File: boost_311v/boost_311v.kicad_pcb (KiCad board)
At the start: 2 copper layers, 44 parts, among them Q1 BC556, Q2 PN2222A, Q3 PN2222A, U1 NE555, U2 4N25, U3 4N25, U4 TL081, U5 NE555

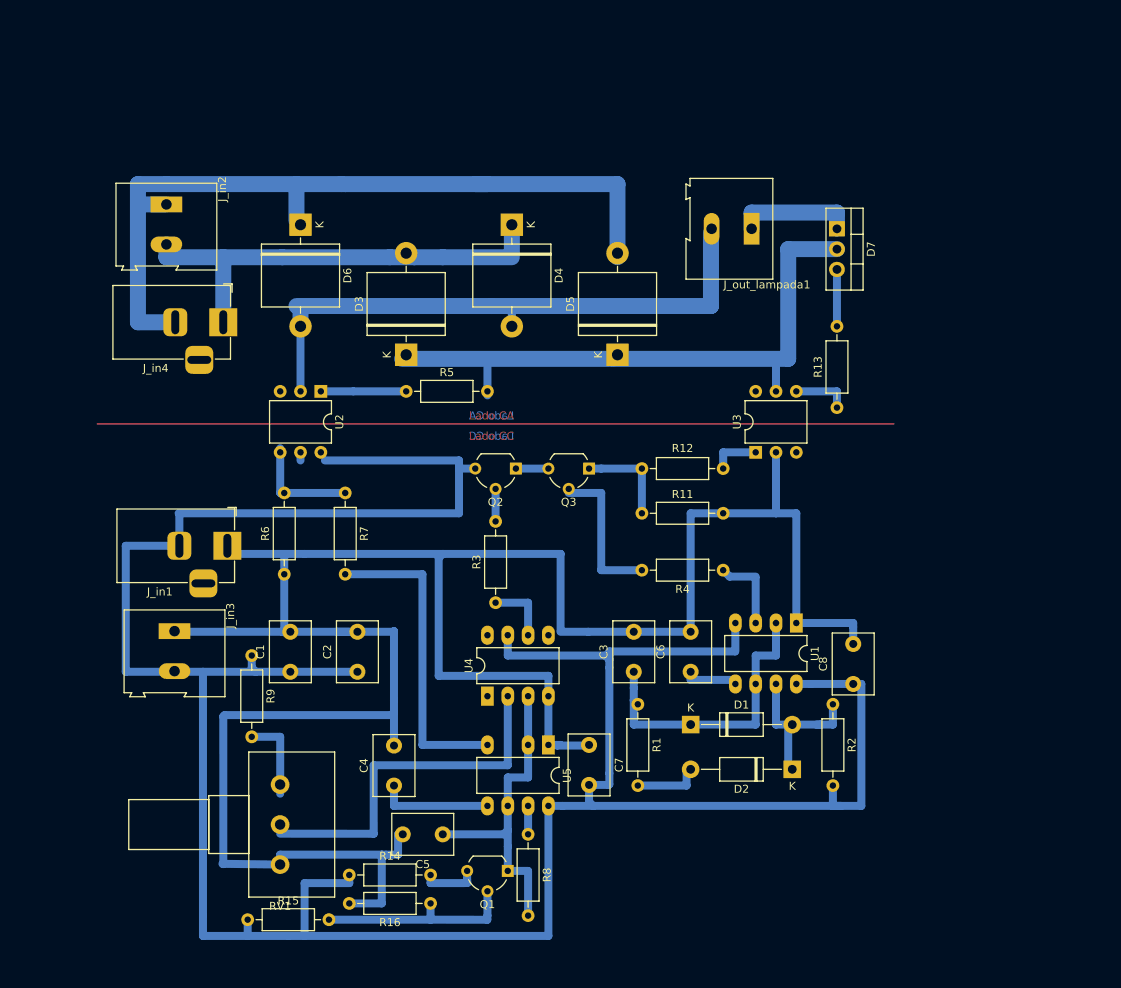
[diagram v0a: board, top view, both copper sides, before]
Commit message: Up pcb
Signed-off-by: fgl27 <fglfgl27@gmail.com>
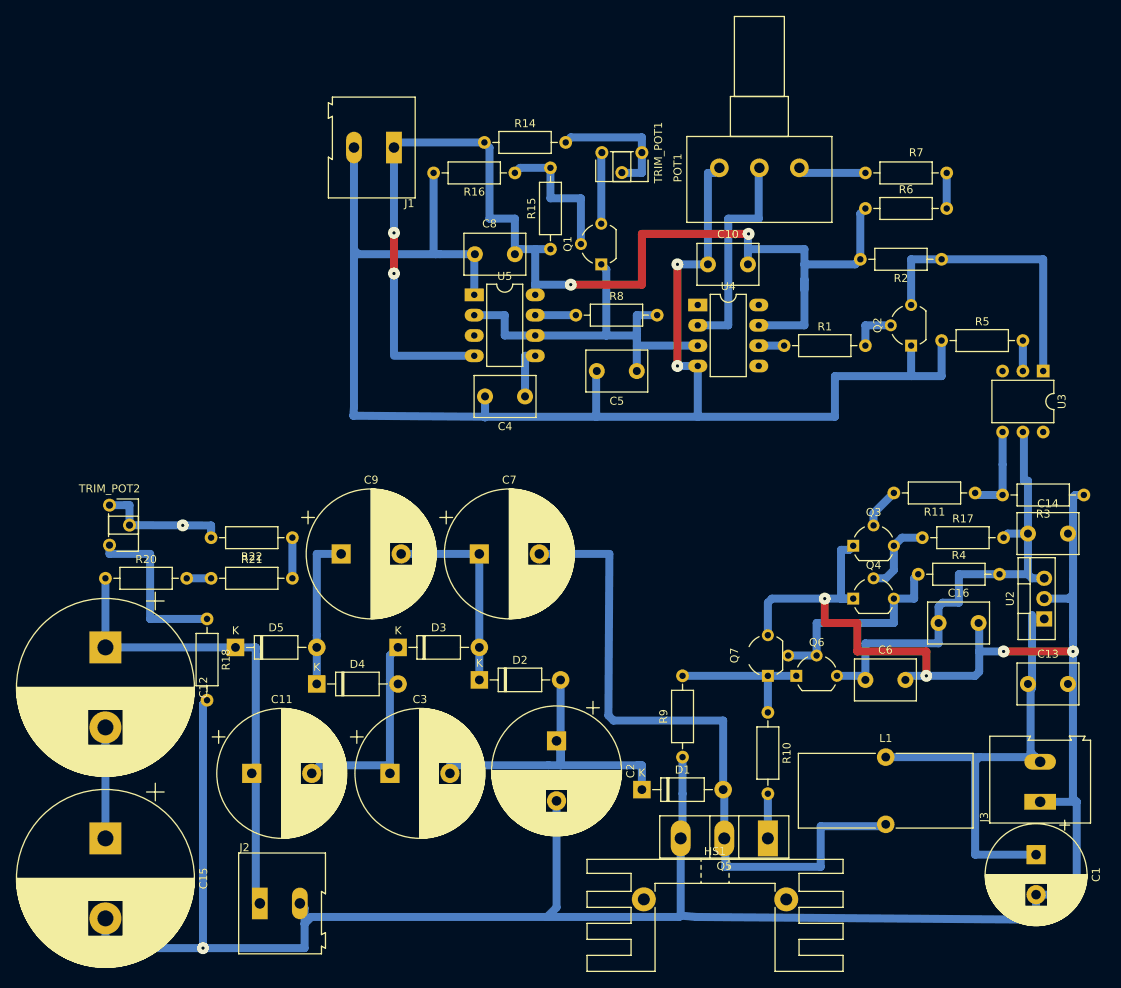
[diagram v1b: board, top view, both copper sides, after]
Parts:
- removed D6: DIODE, Diode_THT:D_5KP_P12.70mm_Horizontal
- removed D7: BT151, Package_TO_SOT_THT:TO-220-3_Vertical
- removed J_in1, J_in4: Screw_Terminal_01x02, Connector_BarrelJack:BarrelJack_Horizontal
- removed J_in2, J_in3, J_out_lampada1: Screw_Terminal_01x02, TerminalBlock:TerminalBlock_Altech_AK300-2_P5.00mm
- removed R12, R13: 1k, Resistor_THT:R_Axial_DIN0207_L6.3mm_D2.5mm_P10.16mm_Horizontal
- removed RV1: POT_10k, Potentiometer_THT:Potentiometer_Alps_RK163_Single_Horizontal
- removed U1: NE555, Package_DIP:DIP-8_W7.62mm_LongPads
- added C10: 100nF, Capacitor_THT:C_Disc_D7.5mm_W5.0mm_P5.00mm, F.Cu at (127.1, 98.4)
- added C11: 100µF_200V, Capacitor_THT:CP_Radial_D16.0mm_P7.50mm, F.Cu at (70.1, 162.1)
- added C12: 200µF_200V, Capacitor_THT:CP_Radial_D22.0mm_P10.00mm_SnapIn, F.Cu at (51.8, 146.3)
- added C13: 10µF, Capacitor_THT:C_Disc_D7.5mm_W5.0mm_P5.00mm, F.Cu at (167.1, 150.9)
- added C14: 100nF, Capacitor_THT:C_Disc_D7.5mm_W5.0mm_P5.00mm, F.Cu at (167.1, 132.1)
- added C15: 200µF_200V, Capacitor_THT:CP_Radial_D22.0mm_P10.00mm_SnapIn, F.Cu at (51.8, 170.2)
- added C16: 100nF, Capacitor_THT:C_Disc_D7.5mm_W5.0mm_P5.00mm, F.Cu at (156.0, 143.3)
- added C9: 100µF_200V, Capacitor_THT:CP_Radial_D16.0mm_P7.50mm, F.Cu at (81.3, 134.6)
- added HS1: Heatsink, Heatsink:Heatsink_Stonecold_HS-132_32x14mm_2xFixation1.5mm, F.Cu at (128.0, 177.8)
- added J1: Vin_cnt, TerminalBlock:TerminalBlock_Altech_AK300-2_P5.00mm, F.Cu at (87.9, 83.8)
- added J2: VO, TerminalBlock:TerminalBlock_Altech_AK300-2_P5.00mm, F.Cu at (71.1, 178.3)
- added J3: Vin_boost, TerminalBlock:TerminalBlock_Altech_AK300-2_P5.00mm, F.Cu at (168.7, 165.6)
- added L1: 20µH, Inductor_THT:L_Toroid_Vertical_L21.6mm_W9.1mm_P8.40mm_Bourns_5700, F.Cu at (149.4, 160.0)
- added POT1: 200kΩ, Potentiometer_THT:Potentiometer_Alps_RK163_Single_Horizontal, F.Cu at (138.6, 86.4)
- added Q4: PN2222A, Package_TO_SOT_THT:TO-92_Wide, F.Cu at (145.3, 140.2)
- added Q5: IRFP260, Package_TO_SOT_THT:TO-247-3_Vertical, F.Cu at (134.6, 170.2)
- added Q6: 2N3904, Package_TO_SOT_THT:TO-92_Wide, F.Cu at (138.2, 149.9)
- added Q7: 2N3906, Package_TO_SOT_THT:TO-92_Wide, F.Cu at (134.6, 149.9)
- added R10: 47Ω, Resistor_THT:R_Axial_DIN0207_L6.3mm_D2.5mm_P10.16mm_Horizontal, F.Cu at (134.6, 154.4)
- added R17: 10kΩ, Resistor_THT:R_Axial_DIN0207_L6.3mm_D2.5mm_P10.16mm_Horizontal, F.Cu at (153.9, 132.6)
- added R18: 100kΩ, Resistor_THT:R_Axial_DIN0207_L6.3mm_D2.5mm_P10.16mm_Horizontal, F.Cu at (64.5, 142.7)
- added R20: 330kΩ, Resistor_THT:R_Axial_DIN0207_L6.3mm_D2.5mm_P10.16mm_Horizontal, F.Cu at (51.8, 137.7)
- added R21: 330kΩ, Resistor_THT:R_Axial_DIN0207_L6.3mm_D2.5mm_P10.16mm_Horizontal, F.Cu at (65.0, 137.7)
- added R22: 220kΩ, Resistor_THT:R_Axial_DIN0207_L6.3mm_D2.5mm_P10.16mm_Horizontal, F.Cu at (75.2, 132.6)
- added TRIM_POT1: 22kΩ, Potentiometer_THT:Potentiometer_ACP_CA6-H2,5_Horizontal, F.Cu at (118.9, 84.5)
- added TRIM_POT2: 22kΩ, Potentiometer_THT:Potentiometer_ACP_CA6-H2,5_Horizontal, F.Cu at (52.3, 128.5)
- C1: value 100n -> 100µF; footprint Capacitor_THT:C_Disc_D7.5mm_W5.0mm_P5.00mm -> Capacitor_THT:CP_Radial_D12.5mm_P5.00mm
- C2: value 100n -> 100µF; footprint Capacitor_THT:C_Disc_D7.5mm_W5.0mm_P5.00mm -> Capacitor_THT:CP_Radial_D16.0mm_P7.50mm
- C3: value 4.7n -> 100µF_200V; footprint Capacitor_THT:C_Disc_D7.5mm_W5.0mm_P5.00mm -> Capacitor_THT:CP_Radial_D16.0mm_P7.50mm
- C4: value 10n -> 10nF
- C5: value 100n -> 500pF
- C6: value 10n -> 100nF
- C7: value 100n -> 100µF_200V; footprint Capacitor_THT:C_Disc_D7.5mm_W5.0mm_P5.00mm -> Capacitor_THT:CP_Radial_D16.0mm_P7.50mm
- C8: value 100n -> 100nF
- D1, D2: value DIODE -> FR154; footprint Diode_THT:D_DO-41_SOD81_P12.70mm_Horizontal -> Diode_THT:D_DO-41_SOD81_P10.16mm_Horizontal
- D3, D4, D5: value DIODE -> FR154; footprint Diode_THT:D_5KP_P12.70mm_Horizontal -> Diode_THT:D_DO-41_SOD81_P10.16mm_Horizontal
- R1: value 2.2k -> 1kΩ
- R11: value 470 -> 10kΩ
- R14: value 10k -> 1kΩ
- R15, R9: value 10k -> 10kΩ
- R16: value 100k -> 100kΩ
- R2: value 1k -> 1kΩ
- R3: value 22k -> 330Ω
- R4: value 22k -> 1kΩ
- R5: value 1k -> 470Ω
- R6: value 40k -> 100kΩ
- R7: value 1k -> 50kΩ
- R8: value 470 -> 330Ω
- U2: value 4N25 -> L7812; footprint Package_DIP:DIP-6_W7.62mm -> Package_TO_SOT_THT:TO-220-3_Vertical
- U4: value TL081 -> LF357
- moved C1 96.0 mm to (168.1, 172.2), turned to 270 degrees
- moved U2 94.8 mm to (169.2, 142.7), turned to 90 degrees
- moved R14 93.1 mm to (99.2, 83.2)
- moved R15 92.0 mm to (107.4, 96.5), turned to 90 degrees
- moved R16 91.9 mm to (103.0, 87.0)
- moved R6 85.8 mm to (146.8, 91.4), turned to 0 degrees
- moved R7 85.2 mm to (157.0, 87.0), turned to 180 degrees
- moved Q1 76.7 mm to (113.8, 98.4), turned to 90 degrees
- moved R3 74.8 mm to (174.1, 127.3), turned to 180 degrees
- moved C8 68.4 mm to (103.0, 97.2), turned to 180 degrees
- moved R5 67.2 mm to (156.3, 108.0)
- moved R8 65.2 mm to (110.6, 104.8), turned to 0 degrees
- moved C5 62.8 mm to (118.2, 111.8)
- moved D4 62.4 mm to (78.2, 150.9), turned to 0 degrees
- moved D5 60.2 mm to (68.1, 146.3), turned to 0 degrees
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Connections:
- net /F_out_Serra renamed /F_Serra
- C1 pad 1: +12V -> +24V
- C1 pad 2: GND -> GND2
- C2 pad 1: +12V -> Net-(C2-Pad1)
- C2 pad 2: GND -> GND2
- C3 pad 1: Net-(C3-Pad1) -> Net-(C11-Pad2)
- C3 pad 2: GND -> Net-(C2-Pad1)
- C4 pad 2: GND -> GND1
- C5 pad 2: GND -> GND1
- C6 pad 1: Net-(C6-Pad1) -> /12V_L7812
- C6 pad 2: GND -> GND2
- C7 pad 1: GND -> Net-(C7-Pad1)
- C7 pad 2: +12V -> Net-(C7-Pad2)
- C8 pad 2: GND -> GND1
- D1 pad 1: Net-(D1-Pad1) -> Net-(C7-Pad2)
- D1 pad 2: Net-(C3-Pad1) -> Net-(C2-Pad1)
- D2 pad 1: Net-(D2-Pad1) -> Net-(C2-Pad1)
- D2 pad 2: Net-(D1-Pad1) -> Net-(C7-Pad1)
- D3 pad 1: Net-(D3-Pad1) -> Net-(C7-Pad1)
- D3 pad 2: /+AC_Retificado -> Net-(C11-Pad2)
- D4 pad 1: /-AC_Retificado -> Net-(C11-Pad2)
- D4 pad 2: Net-(D3-Pad1) -> Net-(C9-Pad1)
- D5 pad 1: AC -> Net-(C9-Pad1)
- D5 pad 2: /+AC_Retificado -> Net-(C11-Pad1)
- Q2 pad 1: Net-(Q2-Pad1) -> GND1
- Q2 pad 3: +12V -> /PWM
- Q3 pad 1: /F_out_AND -> GND2
- Q3 pad 3: Net-(Q2-Pad1) -> Net-(Q3-Pad3)
- R1 pad 1: Net-(C3-Pad1) -> Net-(R1-Pad1)
- R1 pad 2: Net-(D2-Pad1) -> Net-(Q2-Pad2)
- R11 pad 1: /F_out_AND -> Net-(R11-Pad1)
- R11 pad 2: GND -> Net-(Q3-Pad2)
- R14 pad 2: Net-(Q1-Pad3) -> Net-(R14-Pad2)
- R16 pad 2: GND -> GND1
- R2 pad 1: Net-(D1-Pad1) -> /PWM
- R3 pad 1: /F_out_PWM -> GND2
- R3 pad 2: Net-(Q2-Pad2) -> Net-(R11-Pad1)
- R4 pad 1: /F_ataque -> Net-(Q4-Pad3)
- R4 pad 2: Net-(Q3-Pad2) -> /12V_L7812
- R5 pad 1: Net-(R5-Pad1) -> GND1
- R5 pad 2: /+AC_Retificado -> Net-(R5-Pad2)
- R6 pad 1: GND -> +12V
- R7 pad 2: Net-(R7-Pad2) -> Net-(POT1-Pad1)
- R9 pad 1: +12V -> GND2
- R9 pad 2: Net-(R9-Pad2) -> /MOS_Gate
- U2 pad 1: Net-(R5-Pad1) -> +24V
- U2 pad 2: /-AC_Retificado -> GND2
- U2 pad 3: Net-(U2-Pad3) -> /12V_L7812
- U3 pad 1: Net-(R12-Pad1) -> /PWM
- U3 pad 2: GND -> Net-(R5-Pad2)
- U3 pad 4: Net-(R13-Pad1) -> Net-(R11-Pad1)
- U3 pad 5: /+AC_Retificado -> /12V_L7812
- U4 pad 4: GND -> GND1
- U4 pad 6: /F_out_PWM -> Net-(R1-Pad1)
- U5 pad 1: GND -> GND1
- U5 pad 4: Net-(R7-Pad2) -> +12V
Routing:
- net GND2: track 0.00 -> 335.8 mm, vias 0 -> 5
- net GND: track 298.5 -> 0.00 mm
- net +12V: track 349.2 -> 149.4 mm, vias 0 -> 4
- net GND1: track 0.00 -> 198.1 mm, vias 0 -> 2
- net AC: track 102.4 -> 0.00 mm
- net Net-(C7-Pad2): track 0.00 -> 87.2 mm
- net /+AC_Retificado: track 78.1 -> 0.00 mm
- net /-AC_Retificado: track 76.8 -> 0.00 mm
- net +24V: track 0.00 -> 61.3 mm
- net /12V_L7812: track 0.00 -> 60.1 mm
- net Net-(C11-Pad1): track 0.00 -> 59.4 mm
- net Net-(D3-Pad1): track 57.9 -> 0.00 mm
- net Net-(C2-Pad1): track 0.00 -> 39.4 mm
- net Net-(R7-Pad2): track 39.1 -> 0.00 mm
- net Net-(C3-Pad1): track 37.8 -> 0.00 mm
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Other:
- board text removed: "Lado CA"
- board text removed: "Lado CC"
